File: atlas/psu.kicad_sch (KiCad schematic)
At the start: 43 parts, among them U201 TLS115D0EJ, U202 TLS115D0EJ, U203 TLS115D0EJ, U204 TPS70933DBV, U205 LMR14020

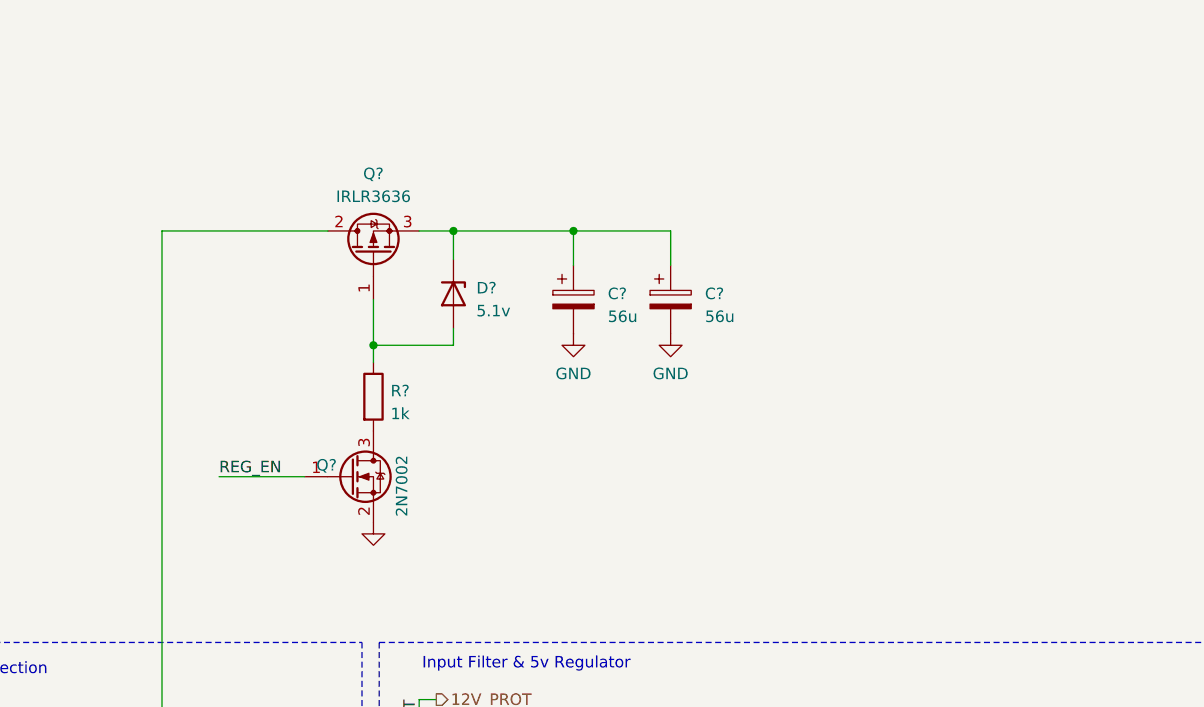
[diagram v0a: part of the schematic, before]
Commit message: hellen modules
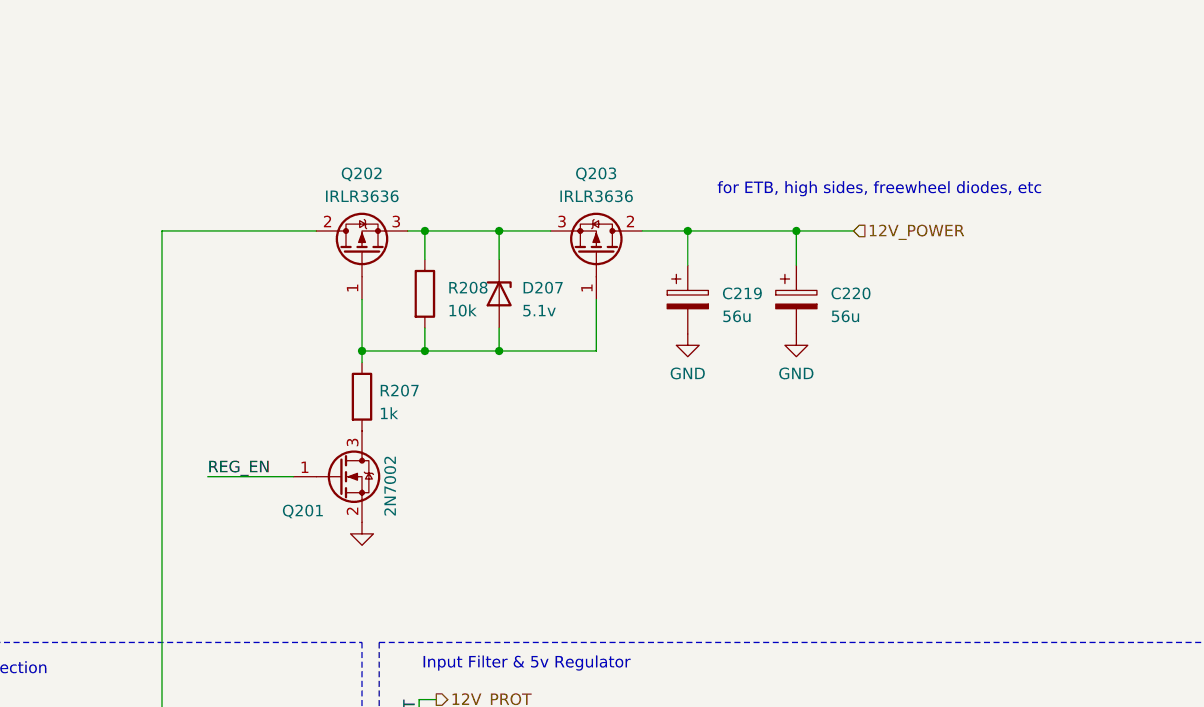
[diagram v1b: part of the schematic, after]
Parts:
- added Q203: IRLR3636, Package_TO_SOT_SMD:TO-252-2, symbol Device:Q_PMOS_GDS
- added R208: 10k, symbol Device:R
- Q202: renamed from Q?; footprint (none) -> Package_TO_SOT_SMD:TO-252-2
- gave numbers to parts that had none: 5
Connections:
- net at D207.1 (K), Q202.3 (S): now also Q203.3 (S), R208.1; no longer C219.1, C220.1
- net at D207.2 (A), Q202.1 (G), R207.1: now also Q203.1 (G), R208.2
- new net 12V_POWER: C219.1, C220.1, Q203.2 (D)
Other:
- note added: "for ETB, high sides, freewheel diodes, etc"
- moved on the sheet: C219, C220, D207, Q201, Q202, R207
